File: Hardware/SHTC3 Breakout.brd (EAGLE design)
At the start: 25.4 x 25.4 mm, 37 parts, among them J2 QWIIC_RIGHT_ANGLE, J3 PTH, J4 QWIIC_RIGHT_ANGLE, U1 SHTC3

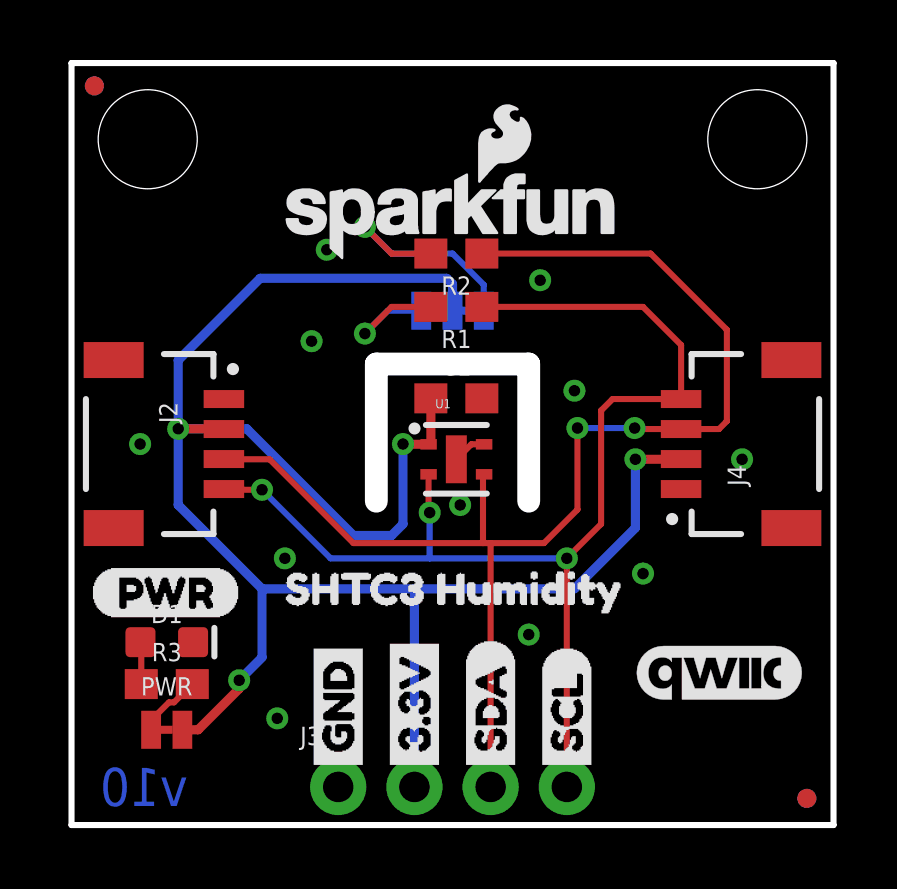
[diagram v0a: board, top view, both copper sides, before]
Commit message: post review/checklist changes, ready for QC double check
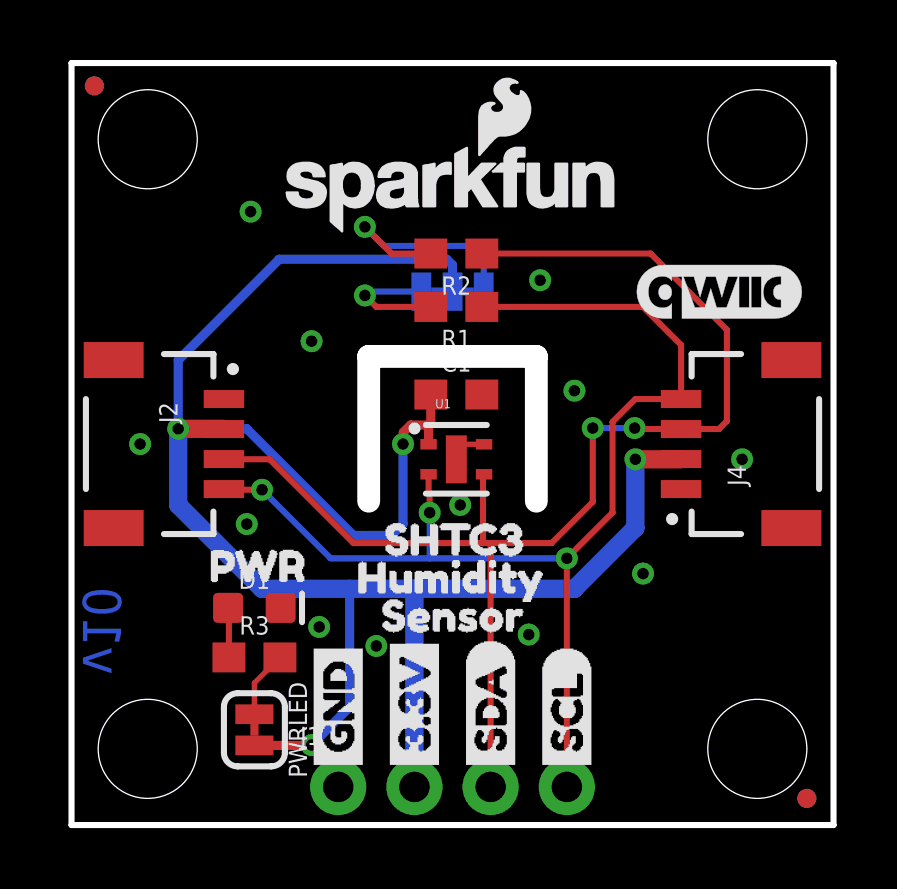
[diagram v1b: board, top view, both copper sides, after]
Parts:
- removed J3: PTH, SparkX:1X04_NO_SILK
- removed PWR: JUMPER-SMT_2_NC_TRACE_NO-SILK, SparkFun-Jumpers:SMT-JUMPER_2_NC_TRACE_NO-SILK
- added J1: (no value), SparkFun-Connectors:1X04_NO_SILK
- added JP7, JP8: STAND-OFF, SparkFun:STAND-OFF
- added PWRLED: JUMPER-SMT_2_NC_TRACE_SILK, SparkFun-Jumpers:SMT-JUMPER_2_NC_TRACE_SILK
- added U$2: (no value), SparkFun-Buzzard:PWR_TO
- U$10: device Labels-0_04:(PWR) -> buzzard_labels:HUMIDITY2
- U$12: device SparkFun-Aesthetics:QWIIC_5.5MM -> buzzard_labels:SENSOR0
- U$7: device buzzard_labels:SHTC3_HUMIDITY1 -> buzzard_labels (3):SHTC3_HUMIDITY_SENSOR2
- U$8: device buzzard_labels:SHTC3_HUMIDITY1 -> buzzard_labels:_SHTC31
- U1: device SHTC3:SHTC3 -> SparkFun-Sensors:SHTC3
- moved U$11 12.7 mm to (21.6, 17.8)
- moved U$12 12.3 mm to (9.40, 6.99), flipped to the top
- moved U$10 8.02 mm to (8.64, 8.26)
- moved U$8 3.36 mm to (9.14, 9.53)
- moved D1 3.14 mm to (6.10, 7.24)
- moved R3 3.05 mm to (6.10, 5.59)
- moved LOGO1 2.99 mm to (5.46, 4.45)
- moved U$7 2.68 mm to (21.7, 9.40)
- moved LOGO2 0.89 mm to (12.7, 21.2)
- moved LOGO3 0.89 mm to (12.7, 21.2)
- moved I2C 0.64 mm to (12.7, 17.8)
- moved U$9 0.64 mm to (14.1, 19.5)
- moved C1 0.13 mm to (12.8, 14.4)
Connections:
- net 3.3V: now also J1.2, PWRLED.2; no longer J3.2, PWR.2
- net GND: now also J1.1; no longer J3.1
- net N$4: now also PWRLED.1; no longer PWR.1
- net SCL: now also J1.4; no longer J3.4
- net SDA: now also J1.3; no longer J3.3
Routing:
- net 3.3V: track 65.6 -> 68.0 mm
- net GND: track 1.13 -> 1.62 mm, vias 11 -> 12
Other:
- outline, holes or cut-outs redrawn
